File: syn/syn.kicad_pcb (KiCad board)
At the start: 2 copper layers, 61 parts, among them J1 AudioJack2, Q1 BC546, Q2 BC546, Q3 BC546, SW1 Gate1, SW2 Gate2, SW3 Range, SW4 Gate3, SW5 Gate3SW, SW6 Wave, SW7 Mod, SW8 Resonance, SW9 Power, U1 MCP6004

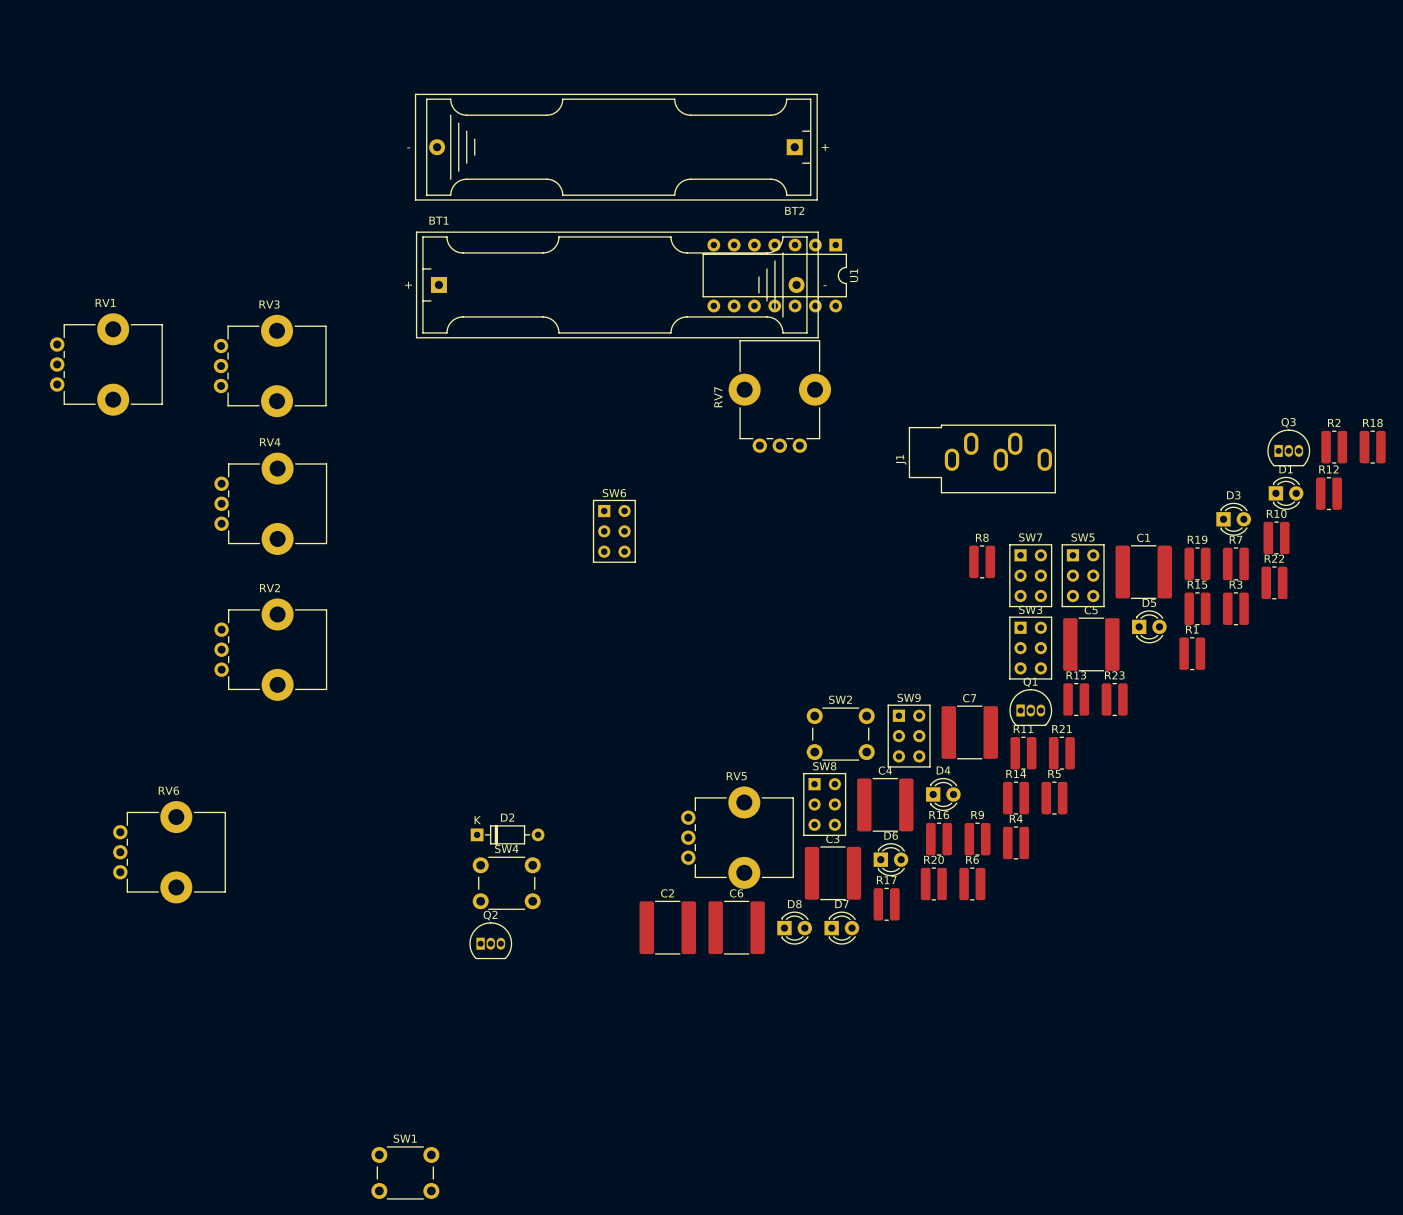
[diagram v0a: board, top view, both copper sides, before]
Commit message: up
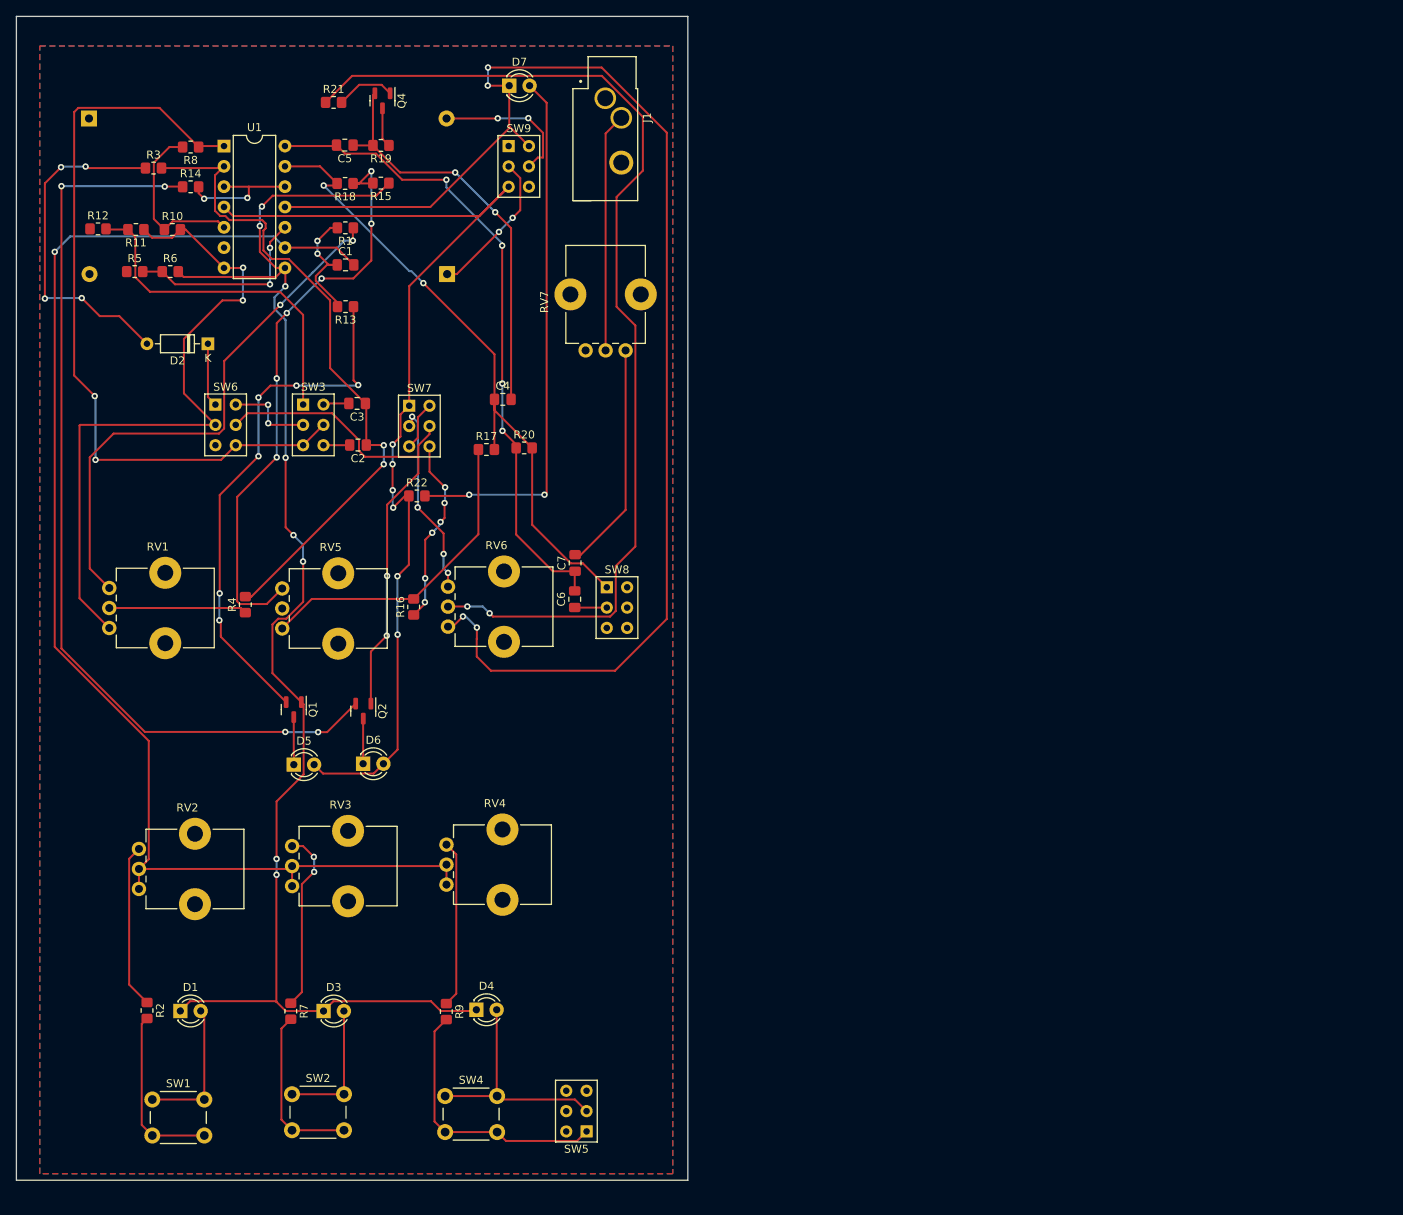
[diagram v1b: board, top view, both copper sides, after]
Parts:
- removed D8: LED, LED_THT:LED_D3.0mm
- removed Q3: BC546, Package_TO_SOT_THT:TO-92_Inline
- removed R23: 470, Resistor_SMD:R_0815_2038Metric_Pad1.20x4.05mm_HandSolder
- added Q4: BC846, Package_TO_SOT_SMD:SOT-23, F.Cu at (81.4, 29.5)
- BT1, BT2: moved to B.Cu
- C1, C2, C3, C4, C5, C6, C7: footprint Capacitor_SMD:C_2225_5664Metric_Pad1.80x6.60mm_HandSolder -> Capacitor_SMD:C_0805_2012Metric_Pad1.18x1.45mm_HandSolder
- J1: value AudioJack2 -> 35RAPC2BV4; footprint Connector_Audio:Jack_3.5mm_CUI_SJ1-3535NG_Horizontal -> 35RAPC2BV4:SWITCHCRAFT_35RAPC2BV4
- Q1, Q2: value BC546 -> BC846; footprint Package_TO_SOT_THT:TO-92_Inline -> Package_TO_SOT_SMD:SOT-23
- R1, R10, R11, R12, R13, R14, R15, R16, R17, R18, R19, R2, R20, R21, R22, R3, R4, R5, R6, R7, R8, R9: footprint Resistor_SMD:R_0815_2038Metric_Pad1.20x4.05mm_HandSolder -> Resistor_SMD:R_0805_2012Metric_Pad1.20x1.40mm_HandSolder
- moved R2 164.3 mm to (52.0, 143.2), turned to -90 degrees
- moved R12 157.4 mm to (45.9, 45.5)
- moved D1 151.5 mm to (56.2, 143.2)
- moved R3 146.1 mm to (52.8, 37.9)
- moved R10 143.3 mm to (55.2, 45.6)
- moved R18 132.6 mm to (76.8, 39.8), turned to 180 degrees
- moved R5 132.5 mm to (50.5, 50.8)
- moved R7 130.7 mm to (70.0, 143.3), turned to -90 degrees
- moved R11 128.8 mm to (50.6, 45.6), turned to 180 degrees
- moved R14 128.4 mm to (57.4, 40.2)
- moved D3 128.2 mm to (74.1, 143.2)
- moved R6 126.1 mm to (54.9, 50.8)
- moved R21 122.1 mm to (75.3, 29.7)
- moved R1 118.5 mm to (76.8, 45.4), turned to 180 degrees
- moved R15 115.1 mm to (81.2, 39.8), turned to 180 degrees
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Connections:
- Q1 pad 1: Net-(D5-Pad1) -> Net-(D1-Pad1)
- Q1 pad 2: Net-(D1-Pad1) -> Net-(Q1-Pad2)
- Q1 pad 3: Net-(Q1-Pad3) -> Net-(D5-Pad1)
- Q2 pad 1: Net-(D6-Pad1) -> Net-(Q2-Pad1)
- Q2 pad 3: Net-(Q2-Pad3) -> Net-(D6-Pad1)
- R13 pad 1: Net-(Q1-Pad3) -> Net-(Q1-Pad2)
- R14 pad 1: Net-(Q2-Pad3) -> Net-(Q2-Pad2)
- RV7 pad 2: Net-(J1-PadT) -> Net-(J1-Pad2)
- SW6 pad 3: unconnected-(SW6-Pad3) -> (no net)
- SW6 pad 5: Net-(Q2-Pad2) -> Net-(Q2-Pad1)
- SW7 pad 5: Net-(Q2-Pad2) -> Net-(Q2-Pad1)
- SW9 pad 1: unconnected-(SW9-Pad1) -> (no net)
- SW9 pad 4: unconnected-(SW9-Pad4) -> (no net)
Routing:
- net Net-(D1-Pad1): track 0.00 -> 179.0 mm, vias 0 -> 8
- net Net-(C1-Pad2): track 0.00 -> 168.3 mm, vias 0 -> 1
- net VSS: track 0.00 -> 167.9 mm, vias 0 -> 4
- net VCC: track 0.00 -> 130.7 mm, vias 0 -> 6
- net Net-(R21-Pad1): track 0.00 -> 130.1 mm, vias 0 -> 2
- net Net-(Q2-Pad2): track 0.00 -> 115.6 mm, vias 0 -> 4
- net TRI_SAW: track 0.00 -> 95.9 mm, vias 0 -> 2
- net Net-(R10-Pad2): track 0.00 -> 85.0 mm, vias 0 -> 2
- net Net-(C2-Pad1): track 0.00 -> 84.0 mm, vias 0 -> 2
- net Net-(C5-Pad2): track 0.00 -> 81.7 mm, vias 0 -> 4
- net Net-(C4-Pad1): track 0.00 -> 81.4 mm, vias 0 -> 2
- net Net-(R15-Pad2): track 0.00 -> 75.0 mm, vias 0 -> 6
- net Net-(R1-Pad1): track 0.00 -> 68.0 mm, vias 0 -> 2
- net Net-(D7-Pad2): track 0.00 -> 67.1 mm, vias 0 -> 2
- net Net-(Q1-Pad2): track 0.00 -> 66.7 mm, vias 0 -> 6
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- added copper zone on B.Cu, net GND
- added copper zone on F.Cu, net GND
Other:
- board outline added: 83.9 x 145.5 mm
